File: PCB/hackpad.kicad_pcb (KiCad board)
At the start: 2 copper layers, 133 x 100 mm, 34 parts, among them J1 OLED_128x64, K1 SW_Push, K2 SW_Push, K3 SW_Push, K4 SW_Push, K5 SW_Push, Q1 SW_Push, T1 SW_Push, U1 XIAO-RP2040-DIP

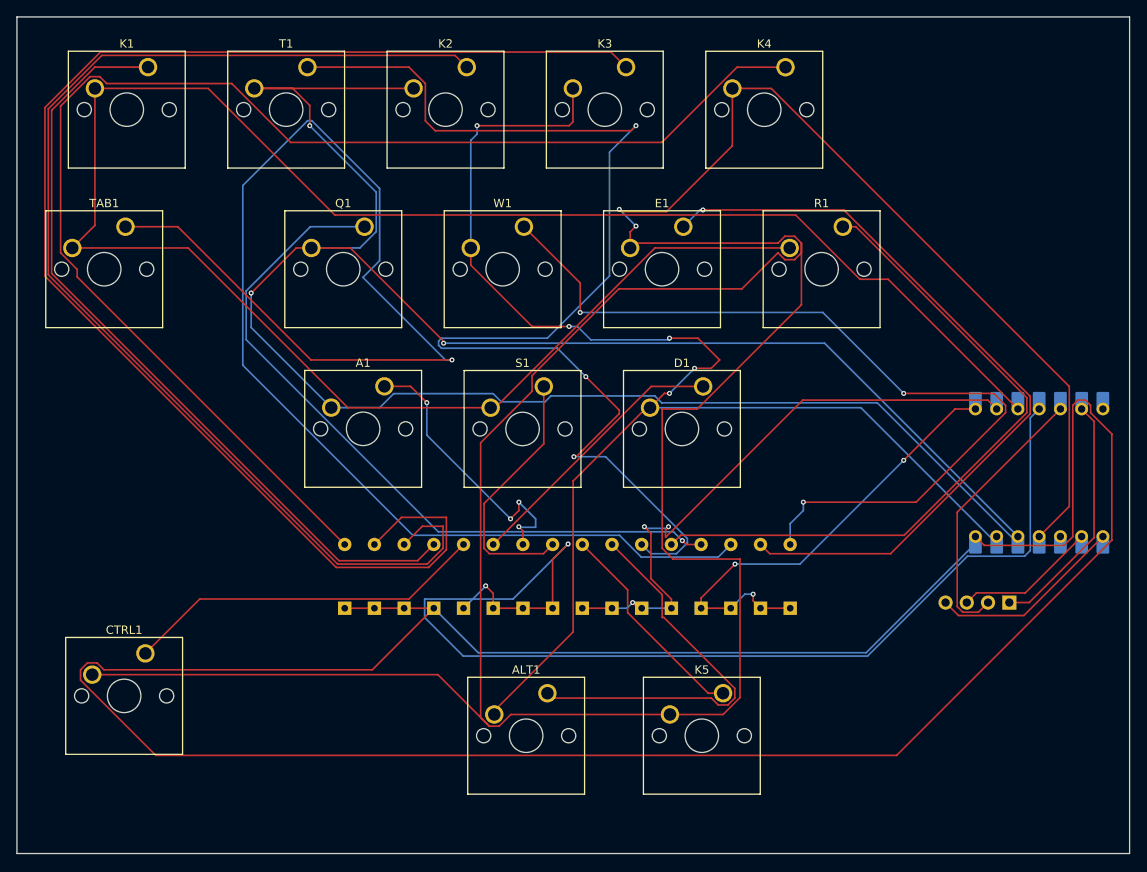
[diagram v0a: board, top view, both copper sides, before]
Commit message: asd
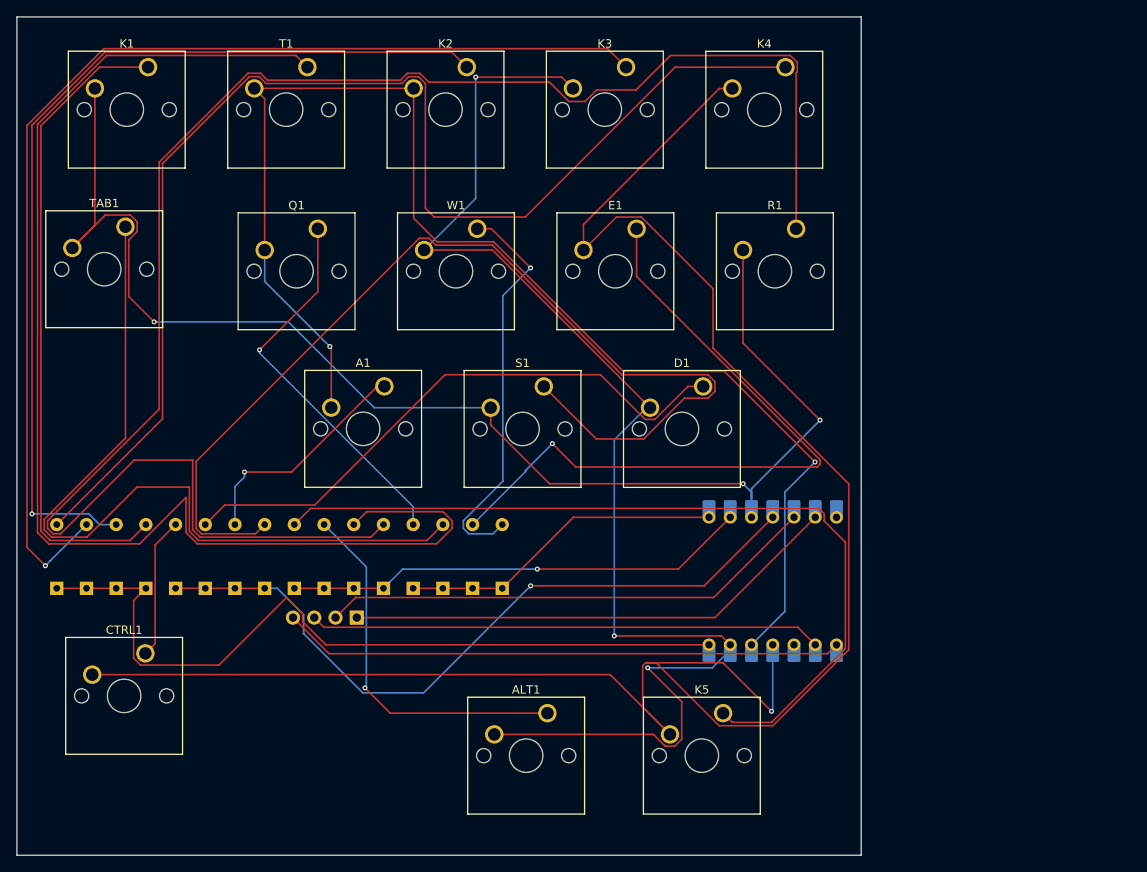
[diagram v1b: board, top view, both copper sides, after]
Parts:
- moved J1 78.0 mm to (47.8, 97.8)
- moved D12 34.5 mm to (40.6, 94.3)
- moved D13 34.5 mm to (37.1, 94.3)
- moved D14 34.5 mm to (33.5, 94.3)
- moved D17 34.5 mm to (22.9, 94.3)
- moved D18 34.5 mm to (19.3, 94.3)
- moved D19 34.5 mm to (15.8, 94.3)
- moved D4 34.5 mm to (69.0, 94.3)
- moved D7 34.5 mm to (58.4, 94.3)
- moved D8 34.5 mm to (54.8, 94.3)
- moved D9 34.5 mm to (51.3, 94.3)
- moved D10 34.5 mm to (47.7, 94.3)
- moved D11 34.5 mm to (44.2, 94.3)
- moved D15 34.5 mm to (30.0, 94.3)
- moved D16 34.5 mm to (26.4, 94.3)
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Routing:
- net Row 0: track 315.9 -> 95.0 mm
- net Column 3: track 363.9 -> 236.8 mm, vias 2 -> 1
- net Net-(D8-A): track 81.3 -> 208.0 mm
- net Column 1: track 270.2 -> 161.6 mm, vias 3 -> 2
- net Net-(D12-A): track 31.2 -> 123.7 mm
- net Net-(D6-A): track 184.7 -> 97.3 mm, vias 1 -> 0
- net Column 0: track 248.0 -> 166.7 mm, vias 0 -> 3
- net Net-(D11-A): track 25.8 -> 100.3 mm
- net Net-(D4-A): track 103.7 -> 48.2 mm, vias 3 -> 1
- net Row 3: track 141.3 -> 86.6 mm, vias 2 -> 1
- net Net-(J1-SCL): track 17.0 -> 61.2 mm
- net Net-(J1-SDA): track 23.4 -> 67.2 mm
- net Net-(D7-A): track 87.7 -> 45.8 mm
- net Net-(D14-A): track 32.9 -> 70.8 mm
- net Net-(D18-A): track 170.2 -> 136.8 mm, vias 0 -> 1
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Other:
- board size 133 x 100 mm -> 100.9 x 100.2 mm
